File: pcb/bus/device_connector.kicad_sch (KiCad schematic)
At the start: 1 part, among them J401 Conn_02x10_Row_Letter_First

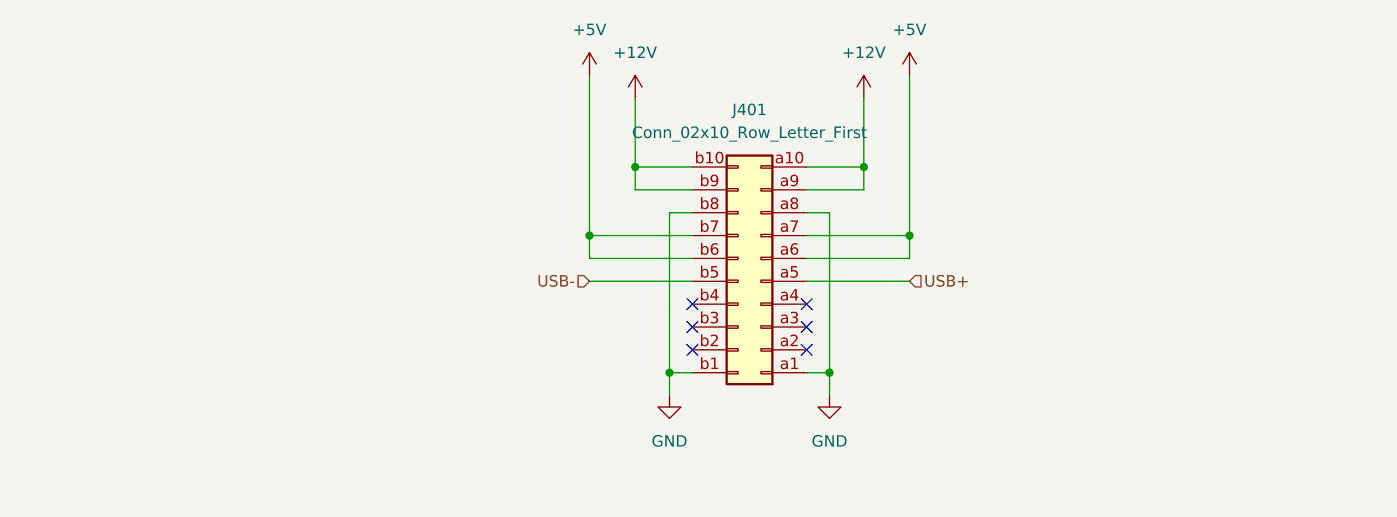
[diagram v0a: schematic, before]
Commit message: update bus pcb
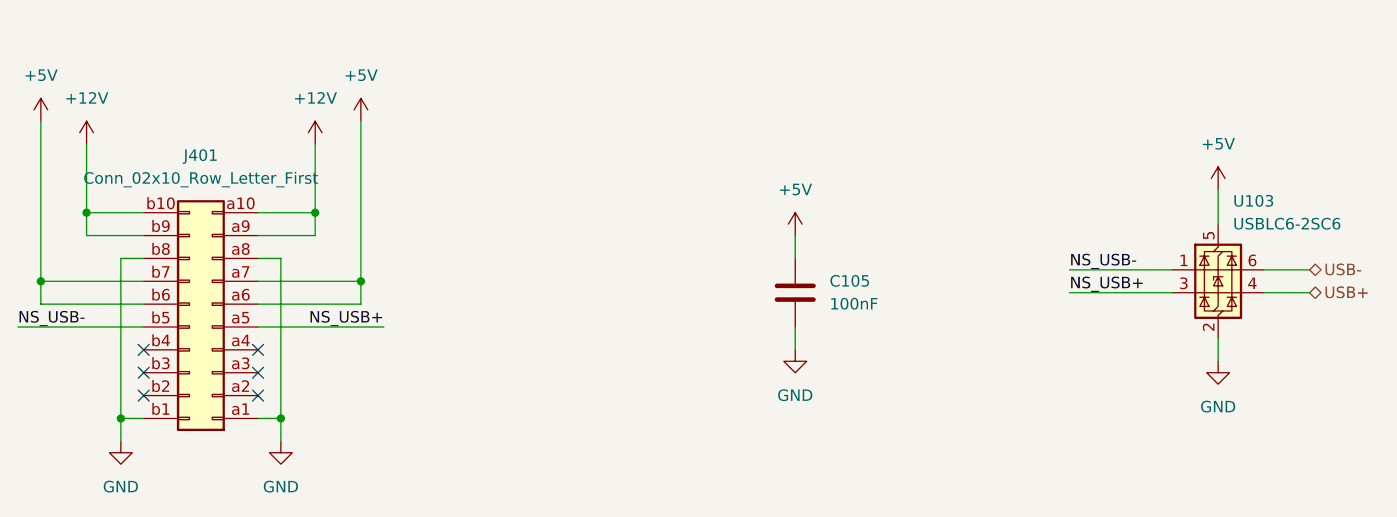
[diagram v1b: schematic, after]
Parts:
- added C105: 100nF, Capacitor_SMD:C_0805_2012Metric, symbol Device:C
- added U103: USBLC6-2SC6, Package_TO_SOT_SMD:SOT-666, symbol Power_Protection:USBLC6-2SC6
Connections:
- net +5V: now also C105.1, U103.5 (VBUS)
- net GND: now also C105.2, U103.2 (GND)
- net USB+: now also U103.4 (I/O2); no longer J401.a5 (Pin_a5)
- net USB-: now also U103.6 (I/O1); no longer J401.b5 (Pin_b5)
- new net NS_USB+: J401.a5 (Pin_a5), U103.3 (I/O2)
- new net NS_USB-: J401.b5 (Pin_b5), U103.1 (I/O1)
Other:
- moved on the sheet: J401
